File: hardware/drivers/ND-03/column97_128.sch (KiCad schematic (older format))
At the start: 24 parts, among them J52 Screw_Terminal_1x02, J53 Screw_Terminal_1x02, J54 Screw_Terminal_1x02, J55 Screw_Terminal_1x02, J56 Screw_Terminal_1x02, J57 Screw_Terminal_1x02, J58 Screw_Terminal_1x02, J59 Screw_Terminal_1x02, J60 Screw_Terminal_1x02, J61 Screw_Terminal_1x02, J62 Screw_Terminal_1x02, J63 Screw_Terminal_1x02, J64 Screw_Terminal_1x02, J65 Screw_Terminal_1x02, J66 Screw_Terminal_1x02, J67 Screw_Terminal_1x02, U16 74HC595, U17 74HC595, U18 74HC595, U19 74HC595

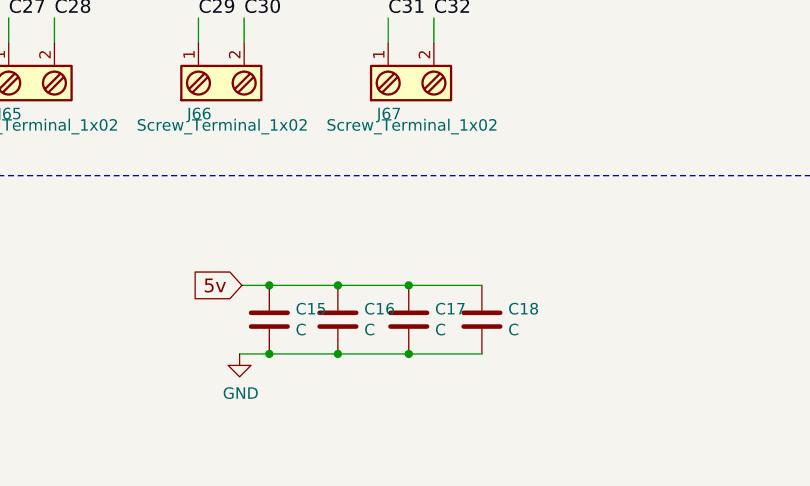
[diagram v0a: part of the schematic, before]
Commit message: Multple commits enclosed in this commit.
1.Design passes all DRC tests.
2.Add PMOS reverse polarity protection on 5v direct input.
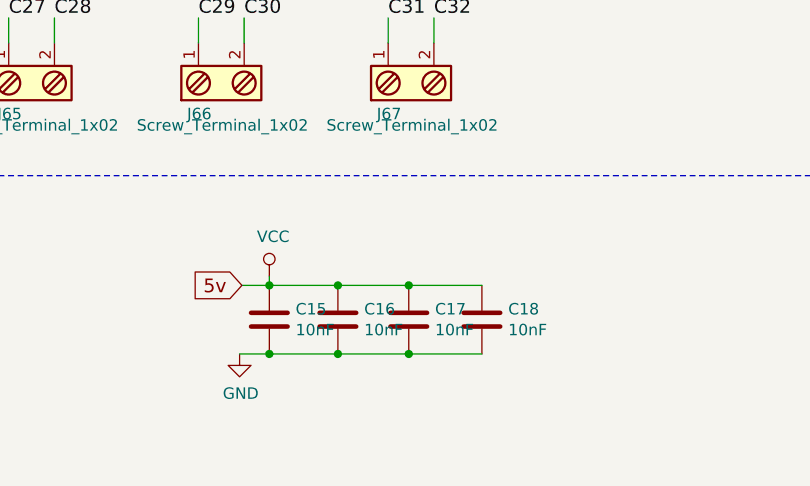
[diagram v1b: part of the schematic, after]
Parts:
- C15, C16, C17, C18: value C -> 10nF
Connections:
- net 5v is gone; now on net VCC: C15.1, C16.1, C17.1, C18.1, U16.10 (SRCLR), U17.10 (SRCLR), U18.10 (SRCLR), U19.10 (SRCLR)
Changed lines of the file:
@@
 5v
 $Comp
-L GND #PWR027
+L GND #PWR031
 U 1 1 599932C1
 P 1660 1810
-F 0 "#PWR027" H 1660 1560 50  0001 C CNN
+F 0 "#PWR031" H 1660 1560 50  0001 C CNN
 F 1 "GND" H 1665 1637 50  0000 C CNN
 F 2 "" H 1660 1810 50  0001 C CNN
@@
 $EndComp
 $Comp
-L GND #PWR028
+L GND #PWR032
 U 1 1 599932C7
 P 3710 1820
-F 0 "#PWR028" H 3710 1570 50  0001 C CNN
+F 0 "#PWR032" H 3710 1570 50  0001 C CNN
 F 1 "GND" H 3715 1647 50  0000 C CNN
 F 2 "" H 3710 1820 50  0001 C CNN
@@
 $EndComp
 $Comp
-L GND #PWR029
+L GND #PWR033
 U 1 1 599932CD
 P 5860 1850
-F 0 "#PWR029" H 5860 1600 50  0001 C CNN
+F 0 "#PWR033" H 5860 1600 50  0001 C CNN
 F 1 "GND" H 5865 1677 50  0000 C CNN
 F 2 "" H 5860 1850 50  0001 C CNN
@@
 $EndComp
 $Comp
-L GND #PWR030
+L GND #PWR034
 U 1 1 599932D3
 P 8120 1840
-F 0 "#PWR030" H 8120 1590 50  0001 C CNN
+F 0 "#PWR034" H 8120 1590 50  0001 C CNN
 F 1 "GND" H 8125 1667 50  0000 C CNN
 F 2 "" H 8120 1840 50  0001 C CNN
@@
 P 2950 7170
 F 0 "C15" H 3065 7216 50  0000 L CNN
-F 1 "C" H 3065 7125 50  0000 L CNN
+F 1 "10nF" H 3065 7125 50  0000 L CNN
 F 2 "Capacitors_THT:C_Disc_D3.4mm_W2.1mm_P2.50mm" H 2988 7020 50  0001 C CNN
 F 3 "" H 2950 7170 50  0001 C CNN
@@
 P 3250 7170
 F 0 "C16" H 3365 7216 50  0000 L CNN
-F 1 "C" H 3365 7125 50  0000 L CNN
+F 1 "10nF" H 3365 7125 50  0000 L CNN
 F 2 "Capacitors_THT:C_Disc_D3.4mm_W2.1mm_P2.50mm" H 3288 7020 50  0001 C CNN
 F 3 "" H 3250 7170 50  0001 C CNN
@@
 P 3560 7170
 F 0 "C17" H 3675 7216 50  0000 L CNN
-F 1 "C" H 3675 7125 50  0000 L CNN
+F 1 "10nF" H 3675 7125 50  0000 L CNN
 F 2 "Capacitors_THT:C_Disc_D3.4mm_W2.1mm_P2.50mm" H 3598 7020 50  0001 C CNN
 F 3 "" H 3560 7170 50  0001 C CNN
@@
 P 3880 7170
 F 0 "C18" H 3995 7216 50  0000 L CNN
-F 1 "C" H 3995 7125 50  0000 L CNN
+F 1 "10nF" H 3995 7125 50  0000 L CNN
 F 2 "Capacitors_THT:C_Disc_D3.4mm_W2.1mm_P2.50mm" H 3918 7020 50  0001 C CNN
 F 3 "" H 3880 7170 50  0001 C CNN
@@
 5v
 $Comp
-L GND #PWR031
+L GND #PWR035
 U 1 1 5999A159
 P 2820 7320
-F 0 "#PWR031" H 2820 7070 50  0001 C CNN
+F 0 "#PWR035" H 2820 7070 50  0001 C CNN
 F 1 "GND" H 2825 7147 50  0000 C CNN
 F 2 "" H 2820 7320 50  0001 C CNN
@@
 Text Notes 6970 7800 2    60   ~ 0
 DECOUPLING CAPS\n
+Wire Wire Line
+	2950 6980 2950 7020
+$Comp
+L VCC #PWR036
+U 1 1 59A68DD1
+P 2950 6980
+F 0 "#PWR036" H 2950 6830 50  0001 C CNN
+F 1 "VCC" H 2967 7153 50  0000 C CNN
+F 2 "" H 2950 6980 50  0001 C CNN
+F 3 "" H 2950 6980 50  0001 C CNN
+	1    2950 6980
+	1    0    0    -1
+$EndComp
 $EndSCHEMATC
